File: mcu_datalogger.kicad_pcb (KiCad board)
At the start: 2 copper layers, 29 parts, among them J1 Conn_01x04_Pin, J2 Conn_01x04_Pin, J3 Conn_01x09_Pin, J4 Conn_02x03_Odd_Even, U1 24LC1025, U2 24LC1025, U3 DS1337S_, U4 ATMEGA328P-AU, Y1 32.768, Y2 16 MHz

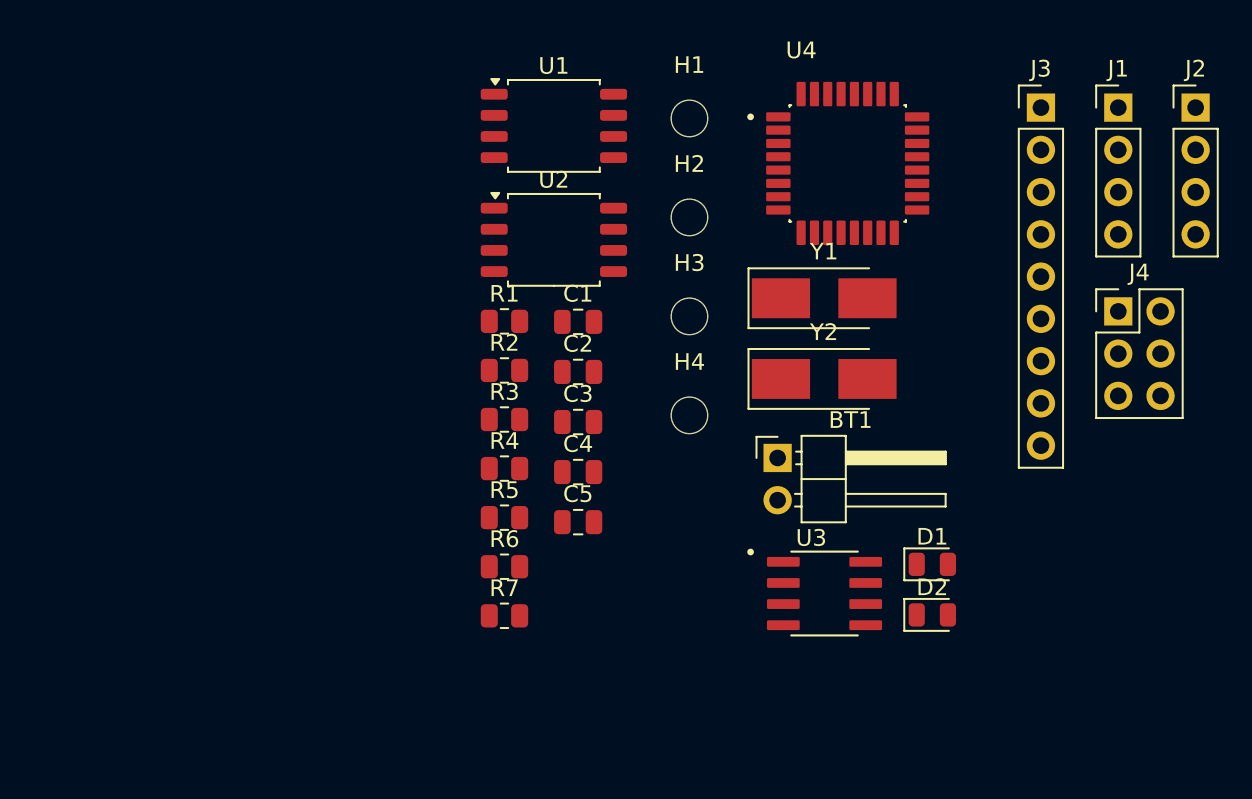
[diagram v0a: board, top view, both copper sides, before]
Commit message: initial pcb layout
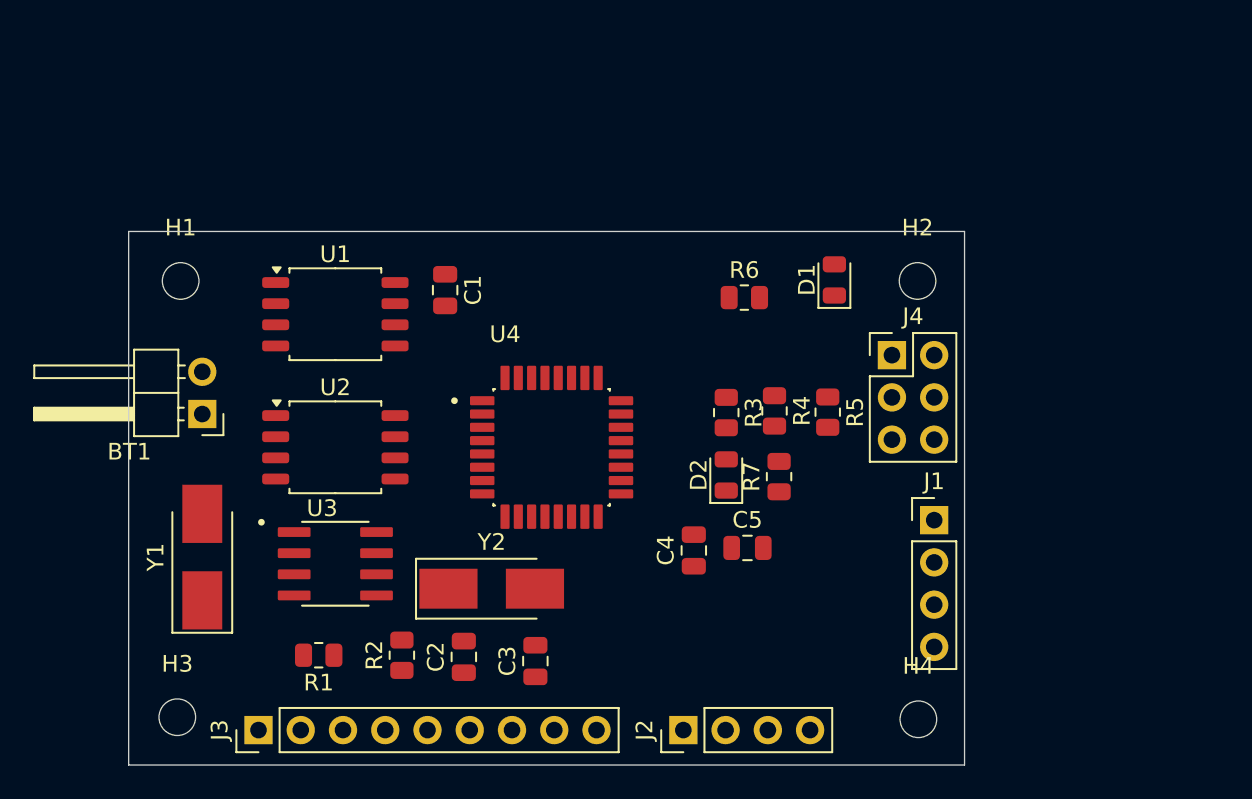
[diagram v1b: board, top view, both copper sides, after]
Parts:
- moved J3 60.1 mm to (105.4, 103.0), turned to 90 degrees
- moved J2 48.5 mm to (130.9, 103.0), turned to 90 degrees
- moved Y1 40.5 mm to (102.0, 92.6), turned to 90 degrees
- moved H3 39.1 mm to (100.5, 102.2)
- moved BT1 34.7 mm to (102.0, 84.0), turned to 180 degrees
- moved H1 32.1 mm to (100.7, 76.0)
- moved U3 29.5 mm to (110.0, 93.0)
- moved J1 27.2 mm to (146.0, 90.4)
- moved U4 24.7 mm to (123.0, 86.0)
- moved Y2 23.6 mm to (119.4, 94.5)
- moved R1 23.0 mm to (109.0, 98.5), turned to 180 degrees
- moved H4 22.9 mm to (145.1, 102.3)
- moved R6 21.7 mm to (134.6, 77.0)
- moved R5 20.4 mm to (139.6, 83.9), turned to -90 degrees
- moved R7 18.5 mm to (136.7, 87.8), turned to 90 degrees
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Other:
- board outline added: 50.2 x 32.1 mm
